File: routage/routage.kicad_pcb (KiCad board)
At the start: 2 copper layers, 110 x 100 mm, 51 parts, among them J2 Conn_01x02, J3 Conn_01x03, Q1 2N2907, Q10 TIP32, Q11 BD138, Q12 TIP31, Q13 2N2222, Q2 2N2907, Q3 2N2907, Q4 2N2222, Q5 2N2222, Q6 2N2907, Q7 2N2907, Q8 BD139, Q9 BD139, U1 Relay_1CT, U2 Jack_Mono

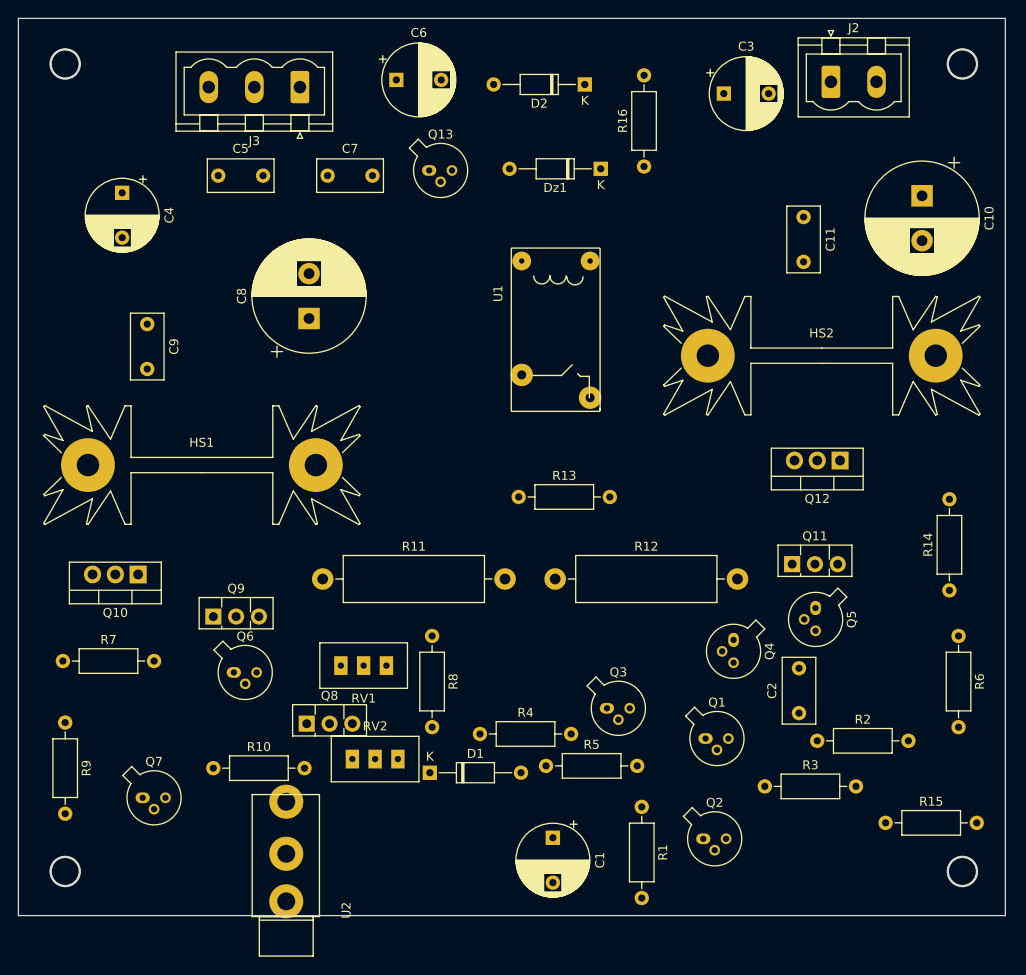
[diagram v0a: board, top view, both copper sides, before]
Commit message: placement corrigé
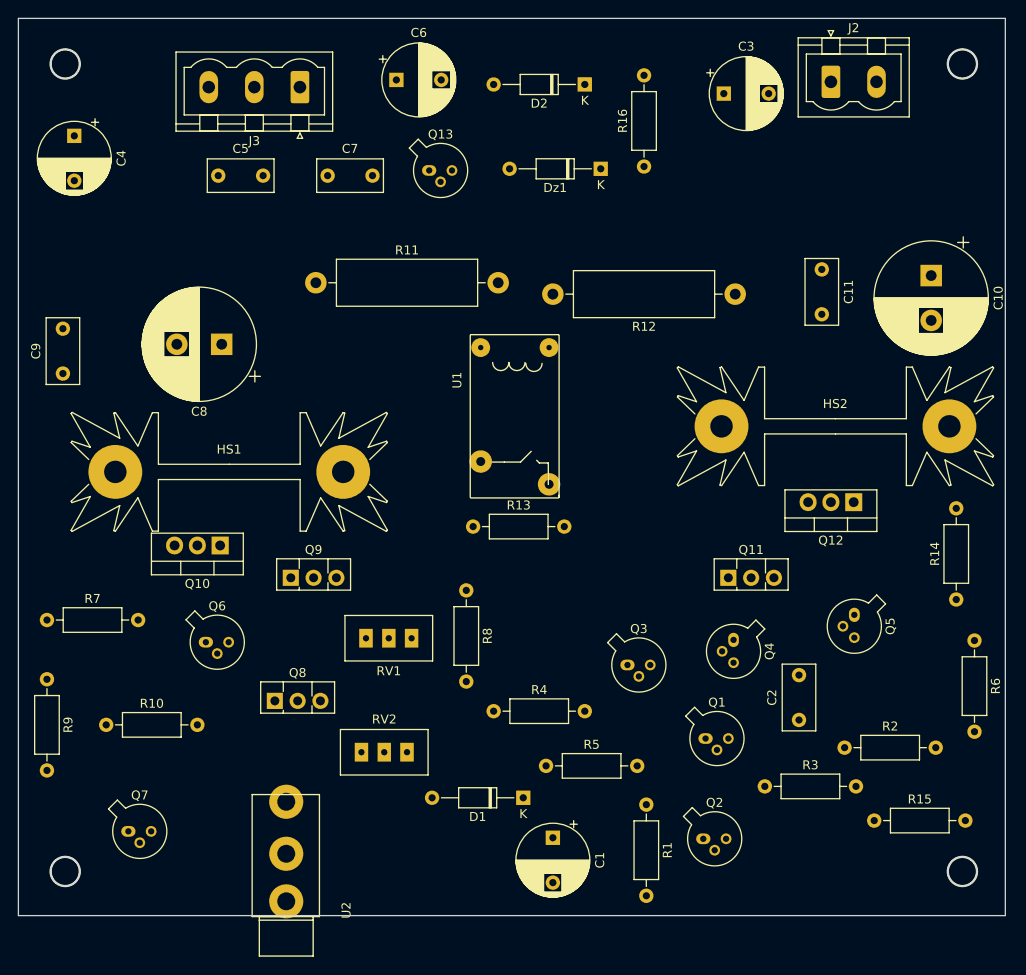
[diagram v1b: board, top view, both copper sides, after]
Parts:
- moved R12 37.6 mm to (170.2, 73.4), turned to 180 degrees
- moved R11 33.0 mm to (123.4, 72.1)
- moved R10 12.9 mm to (100.1, 121.4)
- moved C9 10.9 mm to (95.2, 82.3), turned to 90 degrees
- moved D1 10.8 mm to (146.6, 129.5), turned to 180 degrees
- moved U1 10.7 mm to (132.3, 54.3)
- moved C8 10.1 mm to (113.0, 79.0), turned to 180 degrees
- moved Q10 9.70 mm to (112.8, 101.4)
- moved Q9 9.66 mm to (120.7, 105.0)
- moved C10 8.95 mm to (192.0, 71.3)
- moved C4 8.29 mm to (96.5, 55.8)
- moved HS2 8.02 mm to (181.4, 88.1)
- moved Q11 7.27 mm to (169.4, 105.0)
- moved R8 6.35 mm to (140.2, 106.4)
- moved C11 6.19 mm to (179.8, 70.7)
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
